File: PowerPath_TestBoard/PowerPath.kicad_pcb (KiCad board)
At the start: 2 copper layers, 95.5 x 62.9 mm, 86 parts, among them J1 24V Test, J2 +24V_Ext, J3 12V Test, J4 5V Test, J5 3V Test, J6 +V_in_24V, J7 GND, J8 +Vin_5V, J9 +3V3_Ext, U1 LM76202QPWPRQ1, U2 MCP1826S_LDO, U3 LMR51635XDDCR, U4 LMR51635XDDCR

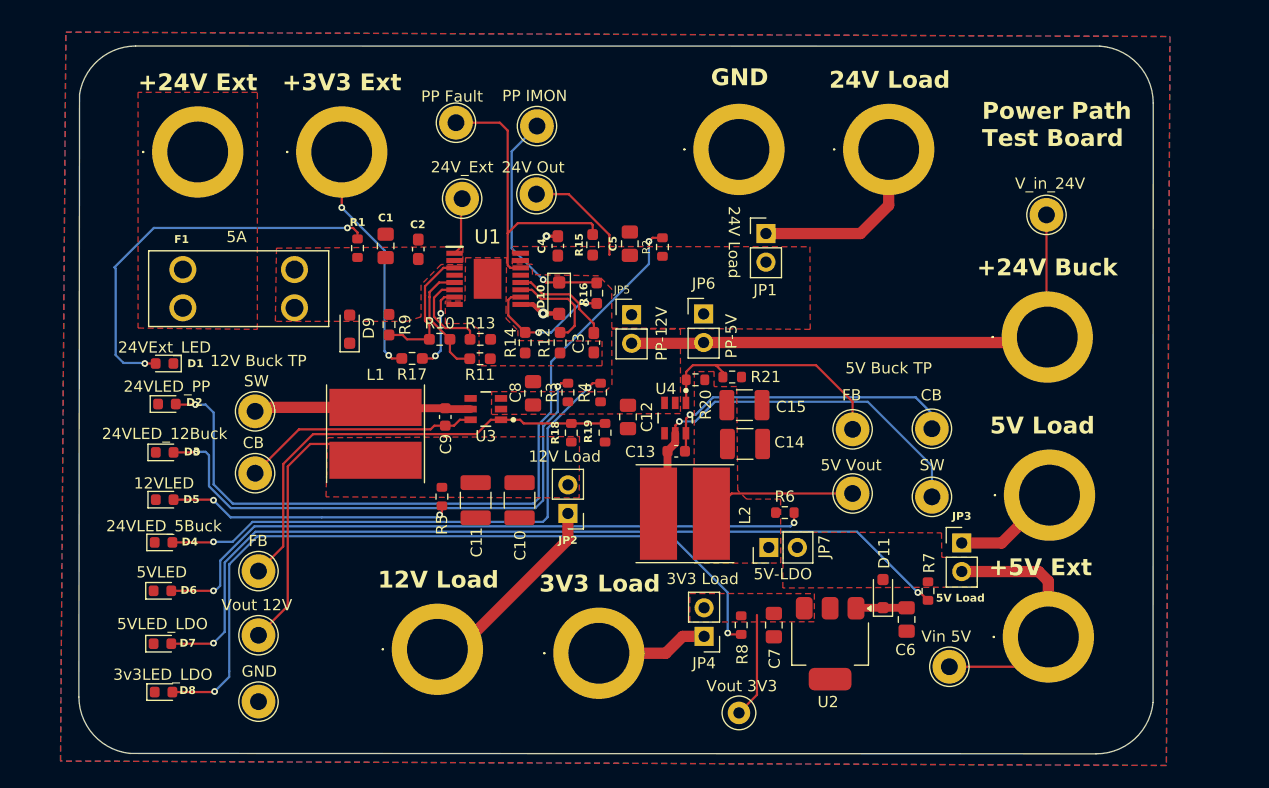
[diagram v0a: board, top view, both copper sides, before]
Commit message: addressed all final comments, review?
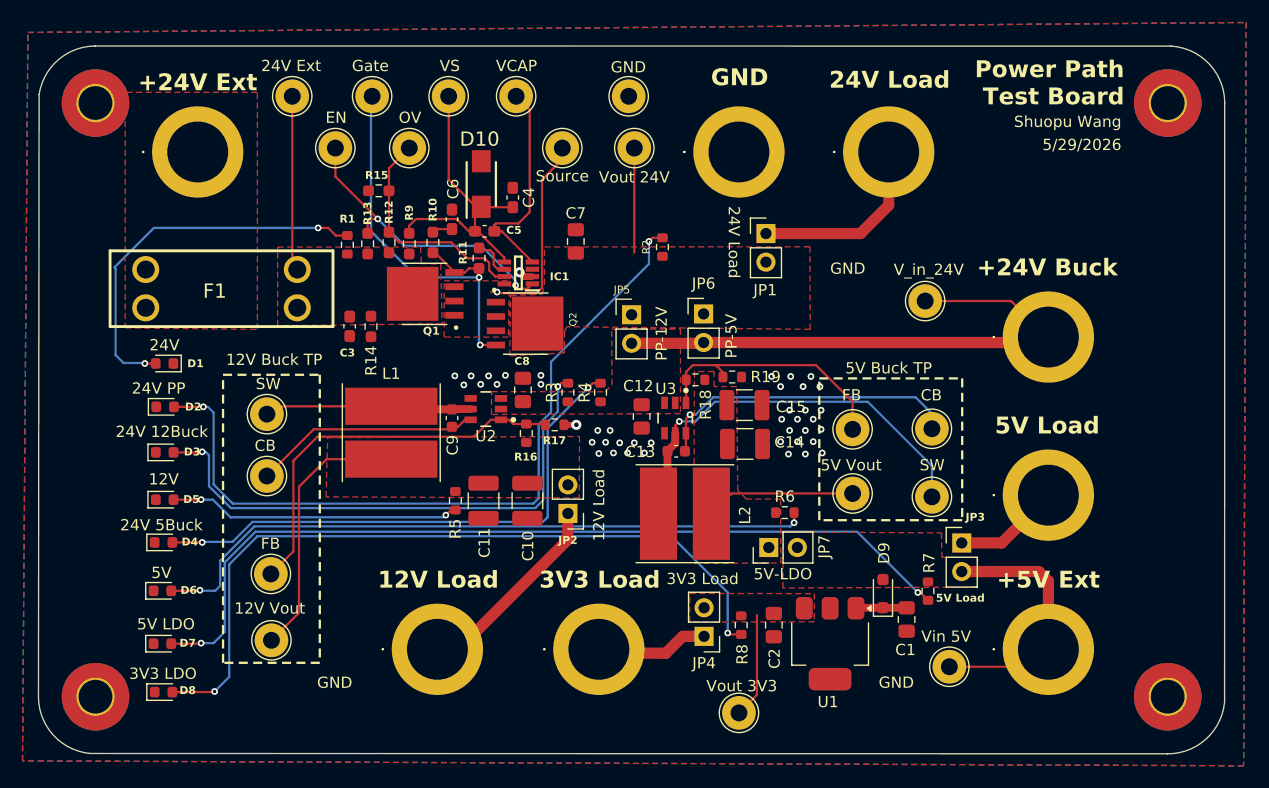
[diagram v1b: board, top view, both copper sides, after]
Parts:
- removed the C1 at (165.6, 79.9)
- removed the C2 at (168.5, 80.2)
- removed the D9 at (162.4, 87.3)
- removed the J9 at (161.7, 71.5)
- removed the R16 at (184.4, 84.1)
- removed the R17 at (167.9, 89.9)
- removed the TP2 at (171.8, 69.0)
- removed the TP3 at (179.1, 69.2)
- removed the U1 at (174.7, 82.8)
- added C6: 10n, Capacitor_SMD:C_0603_1608Metric_Pad1.08x0.95mm_HandSolder, F.Cu at (171.5, 77.5)
- added C7: 10u, Capacitor_SMD:C_0805_2012Metric_Pad1.18x1.45mm_HandSolder, F.Cu at (182.5, 79.5)
- added G***: LHRs_LOGO, UTSVT_Logos:LHRs_LOGO, F.Cu at (224.5, 74.2)
- added G***: LOGO, LOGO, B.Cu at (224.3, 74.2)
- added H1: MountingHole, MountingHole:MountingHole_3mm_Pad_TopBottom, F.Cu at (139.8, 67.2)
- added H2: MountingHole, MountingHole:MountingHole_3mm_Pad_TopBottom, F.Cu at (235.1, 67.2)
- added H3: MountingHole, MountingHole:MountingHole_3mm_Pad_TopBottom, F.Cu at (235.1, 120.0)
- added H4: MountingHole, MountingHole:MountingHole_3mm_Pad_TopBottom, F.Cu at (139.8, 120.0)
- added IC1: LM74502DDFR, UTSVT_Power:SOT65P280X110-8N, F.Cu at (177.4, 82.3)
- added Q1: PSMN012-100YS, PSMN012-100YS:TO127P600X120-5N, F.Cu at (169.1, 84.2)
- added Q2: PSMN012-100YS, PSMN012-100YS:TO127P600X120-5N, F.Cu at (178.1, 86.8)
- added TP14: 24V_OUT, TestPoint:TestPoint_THTPad_D3.0mm_Drill1.5mm, F.Cu at (171.2, 66.6)
- added TP15: 24V_OUT, TestPoint:TestPoint_THTPad_D3.0mm_Drill1.5mm, F.Cu at (164.4, 66.6)
- added TP16: 24V_OUT, TestPoint:TestPoint_THTPad_D3.0mm_Drill1.5mm, F.Cu at (181.3, 71.2)
- added TP17: 24V_OUT, TestPoint:TestPoint_THTPad_D3.0mm_Drill1.5mm, F.Cu at (167.7, 71.2)
- added TP18: 24V_OUT, TestPoint:TestPoint_THTPad_D3.0mm_Drill1.5mm, F.Cu at (161.1, 71.2)
- added TP19: 24V_OUT, TestPoint:TestPoint_THTPad_D3.0mm_Drill1.5mm, F.Cu at (177.2, 66.6)
- C3: value 100nF -> 0.1u
- C4: value 1uF -> 1u
- C5: value 10uF -> 220n; footprint Capacitor_SMD:C_0805_2012Metric_Pad1.18x1.45mm_HandSolder -> Capacitor_SMD:C_0603_1608Metric_Pad1.08x0.95mm_HandSolder
- D10: value TVS -> SMAF4758A; footprint Diode_SMD:D_SOD-123F -> UTSVT_Passives:SODFL5026X125N
- F1: footprint UTSVT_Connectors:FUSE_3568 -> UTSVT_Power:Fuse-3557-2
- R10: value 590 -> 1k
- R11: value 2.1k -> 33
- R12: value 10k -> 223k
- R13: value 402k -> 137k
- R14: value 24m -> 10k
- R9: value 45.3k -> 10k
- TP_3.3V1: footprint TestPoint:TestPoint_Loop_D1.80mm_Drill1.0mm_Beaded -> TestPoint:TestPoint_THTPad_D3.0mm_Drill1.5mm
- moved TP4 63.1 mm to (187.2, 66.6)
- moved C3 21.7 mm to (162.4, 87.0)
- moved R15 19.6 mm to (165.0, 75.0), turned to 180 degrees
- moved TP1 17.6 mm to (157.3, 66.6)
- moved R12 17.6 mm to (165.9, 79.6), turned to 90 degrees
- moved R14 13.8 mm to (164.3, 87.1), turned to 90 degrees
- moved TP7 13.2 mm to (213.6, 84.8)
- moved R13 13.1 mm to (164.0, 79.7), turned to -90 degrees
- moved C5 12.9 mm to (174.4, 78.6), turned to 0 degrees
- moved D10 12.3 mm to (174.1, 74.4), turned to 90 degrees
- moved TP2 9.62 mm to (187.7, 71.2)
- moved R11 8.94 mm to (173.9, 81.0), turned to 90 degrees
- moved R10 8.63 mm to (169.8, 79.6), turned to -90 degrees
- moved R9 7.42 mm to (167.7, 79.7)
- moved C4 5.87 mm to (176.9, 75.6), turned to -90 degrees
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- renumbered C6 to C1, C7 to C2, D11 to D9, J3 to J4, J4 to J5, J5 to J6, J6 to J7, J7 to J8, J8 to J9, R18 to R16, R19 to R17, R20 to R18, R21 to R19, TP12 to TP10, TP14 to TP11, TP15 to TP12, TP16 to TP13, TP4 to TP2, TP5 to TP3, TP6 to TP4, TP7 to TP5, TP8 to TP6, TP9 to TP7, TP10 to TP8, TP11 to TP9, U2 to U1, U3 to U2, U4 to U3
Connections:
- net /PowerProtection/OVP renamed /PowerProtection/gate
- C3 pad 1: Net-(U1-DVDT) -> /+24V_Ext
- C3 pad 2: /PowerProtection/RTN -> GND
- C4 pad 1: /24V_OUT -> GND
- C4 pad 2: GND -> Net-(D10-K)
- C5 pad 1: /24V_OUT -> Net-(D10-K)
- C5 pad 2: GND -> Net-(IC1-VCAP)
- D10 pad 1: /IMON_TP -> Net-(D10-K)
- JP1 pad 2: /24V_OUT -> /Vout_24V
- JP5 pad 1: /24V_OUT -> /Vout_24V
- JP6 pad 1: /24V_OUT -> /Vout_24V
- R10 pad 1: /PowerProtection/UVLO -> Net-(C6-Pad1)
- R11 pad 2: /PowerProtection/RTN -> Net-(IC1-GATE)
- R12 pad 1: /PowerProtection/ILIM -> /+24V_Ext
- R12 pad 2: /PowerProtection/RTN -> Net-(IC1-OV)
- R13 pad 1: /PowerProtection/MODE -> Net-(IC1-EN/UVLO)
- R13 pad 2: /PowerProtection/RTN -> /+24V_Ext
- R14 pad 1: /PowerProtection/IMON -> GND
- R14 pad 2: /PowerProtection/RTN -> /+24V_Ext
- R15 pad 1: /24V_OUT -> Net-(IC1-OV)
- R15 pad 2: /Fault_TP -> GND
- R2 pad 1: /24V_OUT -> /Vout_24V
- R9 pad 1: /+24V_Ext -> Net-(D10-K)
- R9 pad 2: /PowerProtection/UVLO -> /+24V_Ext
- TP2 pad 1: /24V_OUT -> /Vout_24V
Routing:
- net Net-(D10-K): track 0.00 -> 27.6 mm
- net /Fault_TP: track 26.9 -> 0.00 mm
- net Net-(IC1-EN/UVLO): track 0.00 -> 26.7 mm, vias 0 -> 2
- net /PowerProtection/gate: track 10.7 -> 36.7 mm, vias 0 -> 2
- net +3.3V: track 21.1 -> 0.00 mm, vias 2 -> 0
- net /IMON_TP: track 20.6 -> 0.00 mm, vias 1 -> 0
- net Net-(IC1-OV): track 0.00 -> 20.5 mm
- net Net-(IC1-VCAP): track 0.00 -> 19.5 mm
- net /PowerProtection/source: track 0.00 -> 16.3 mm, vias 0 -> 1
- net /PowerProtection/IMON: track 12.2 -> 0.00 mm, vias 2 -> 0
- net /PowerProtection/UVLO: track 11.9 -> 0.00 mm
- net /+24V_Ext: track 5.13 -> 15.6 mm
- net /24V_OUT: track 9.74 -> 0.00 mm
- net Net-(U1-DVDT): track 9.12 -> 0.00 mm
- net /PowerProtection/ILIM: track 8.72 -> 0.00 mm
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- added copper zone on F.Cu, net /PowerProtection/source
- added copper zone on F.Cu, net /Vout_24V
- removed copper zone on F.Cu, net /24V_OUT
- removed copper zone on F.Cu, net /PowerProtection/RTN
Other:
- board size 95.5 x 62.9 mm -> 105.4 x 62.9 mm
- board text added: "12V"
- board text added: "12V Vout"
- board text added: "24V"
- board text added: "24V 12Buck"
- board text added: "24V 5Buck"
- board text added: "24V Ext"
- board text added: "24V PP"
- board text added: "3V3 LDO"
- board text added: "5/29/2026"
- board text added: "5V"
- board text added: "5V LDO"
- board text added: "EN"
- board text added: "Gate"
- board text added: "OV"
- board text added: "Shuopu Wang"
- board text added: "Source"
- board text added: "VCAP"
- board text added: "VS"
- board text added: "Vout 24V"
- board text removed: "+3V3 Ext"
- board text removed: "24V Out"
- board text removed: "PP Fault"
- board text removed: "PP IMON"
- board text removed: "Vout 12V"
